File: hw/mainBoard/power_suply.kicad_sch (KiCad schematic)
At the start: 16 parts, among them Q1 NMOS, Q2 NMOS, U2 LM5148RGYR

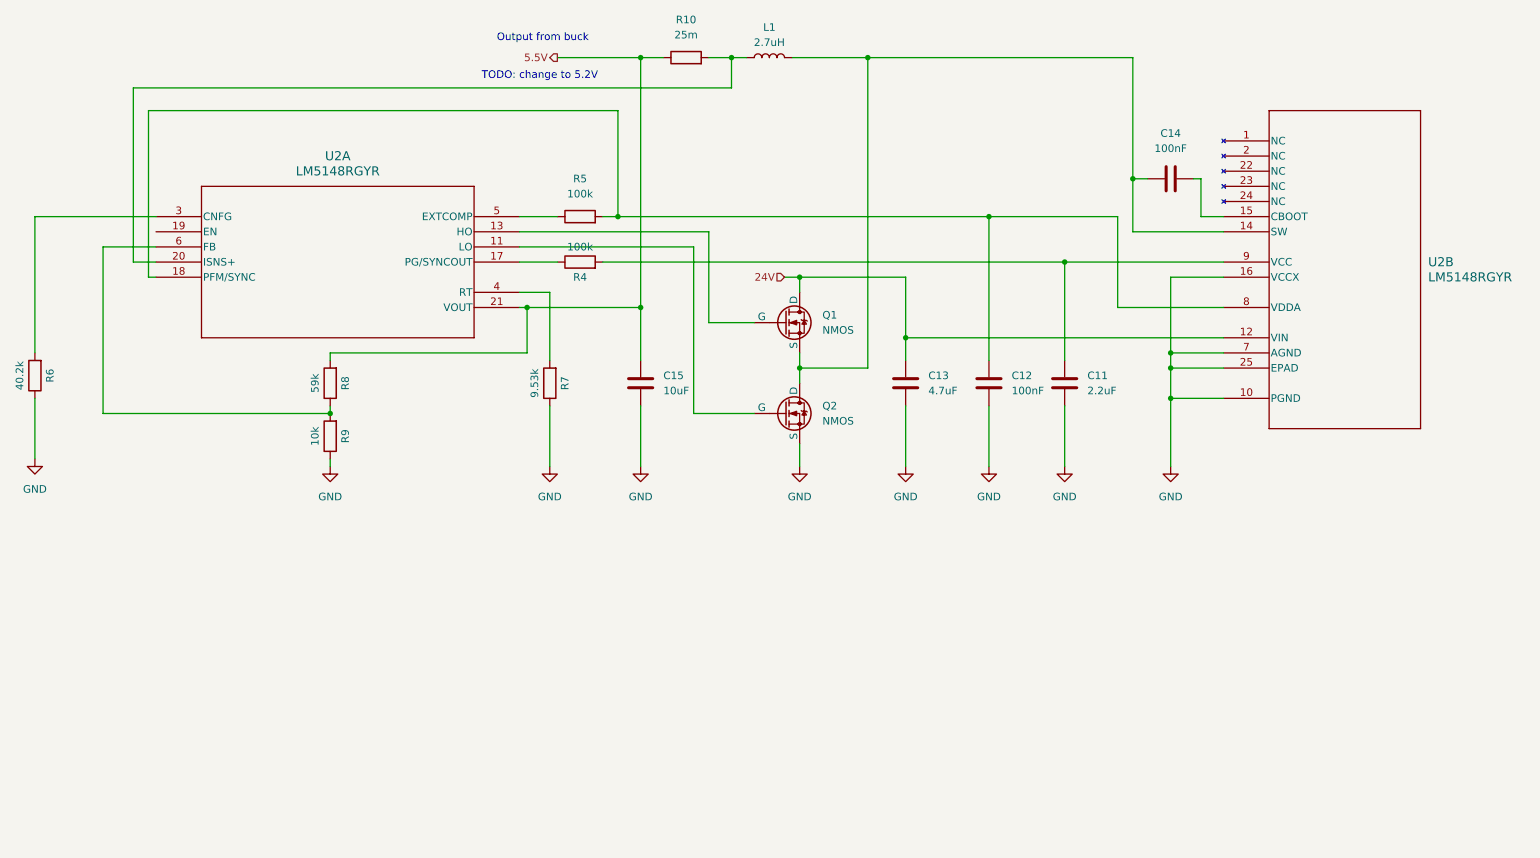
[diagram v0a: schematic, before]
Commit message: schematka
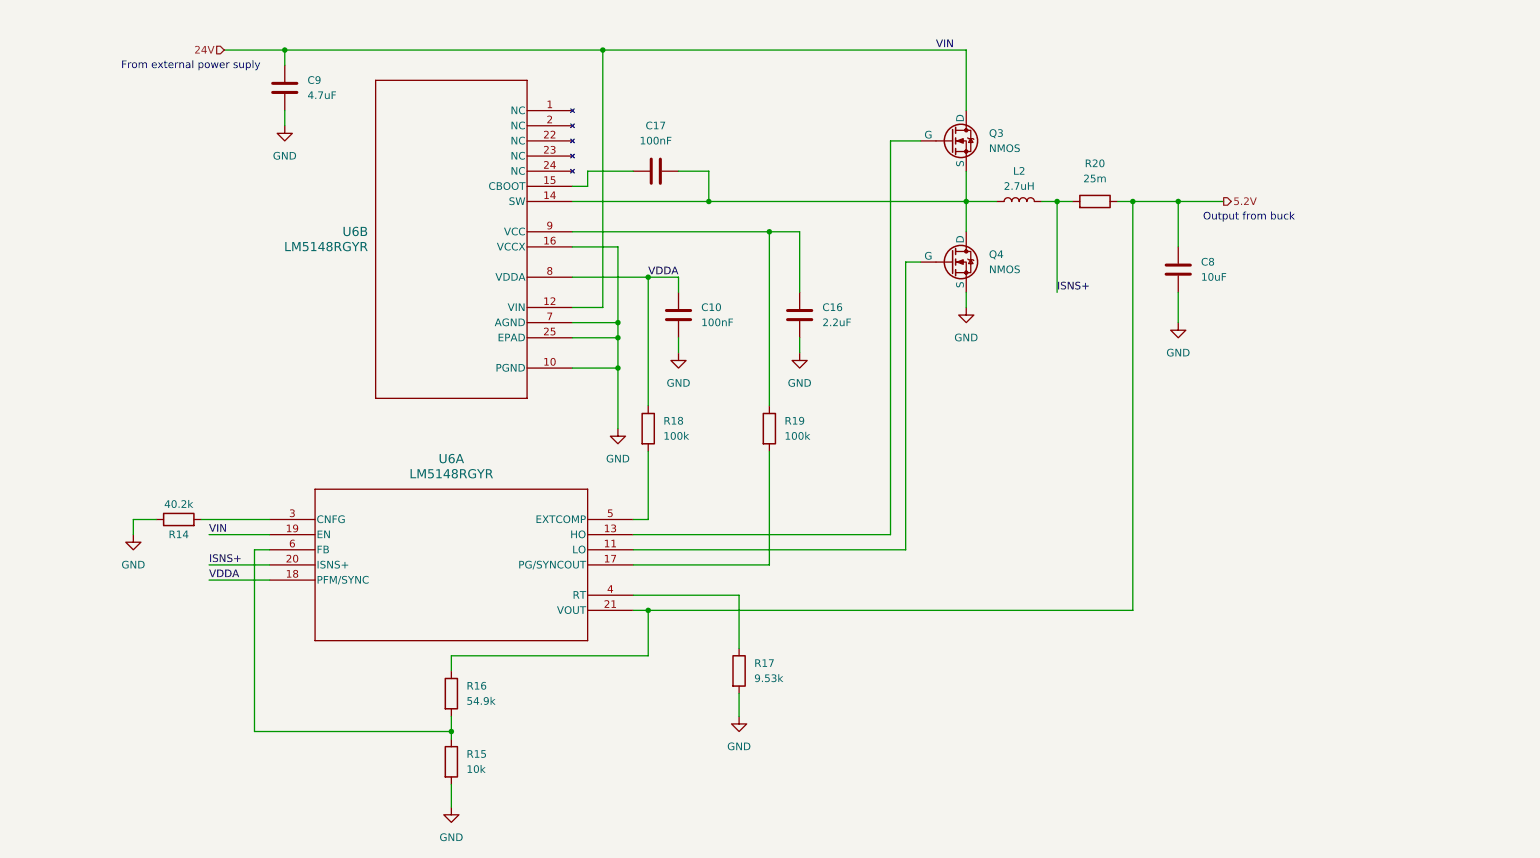
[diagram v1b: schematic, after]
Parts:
- removed C11: 2.2uF, symbol Device:C
- removed C12, C14: 100nF, symbol Device:C
- removed C13: 4.7uF, symbol Device:C
- removed C15: 10uF, symbol Device:C
- removed L1: 2.7uH, symbol Device:L
- removed Q1, Q2: NMOS, symbol Simulation_SPICE:NMOS
- removed R10: 25m, symbol Device:R
- removed R4, R5: 100k, symbol Device:R
- removed R6: 40.2k, symbol Device:R
- removed R7: 9.53k, symbol Device:R
- removed R8: 59k, symbol Device:R
- removed R9: 10k, symbol Device:R
- removed U2: LM5148RGYR, VQFN24_RGY_TEX, symbol LM5148:LM5148RGYR
- added C10, C17: 100nF, symbol Device:C
- added C16: 2.2uF, symbol Device:C
- added C8: 10uF, symbol Device:C
- added C9: 4.7uF, symbol Device:C
- added L2: 2.7uH, symbol Device:L
- added Q3, Q4: NMOS, symbol Simulation_SPICE:NMOS
- added R14: 40.2k, symbol Device:R
- added R15: 10k, symbol Device:R
- added R16: 54.9k, symbol Device:R
- added R17: 9.53k, symbol Device:R
- added R18, R19: 100k, symbol Device:R
- added R20: 25m, symbol Device:R
- added U6: LM5148RGYR, VQFN24_RGY_TEX, symbol LM5148:LM5148RGYR
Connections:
- net 24V: now also C9.1, Q3.1 (D), U6.12 (VIN), U6.19 (EN)
- net GND: now also C10.2, C16.2, C8.2, C9.2, Q4.3 (S), R14.1, R15.2, R17.2, U6.10 (PGND), U6.16 (VCCX), U6.25 (EPAD), U6.7 (AGND)
- new net: C16.1, R19.1, U6.9 (VCC)
- new net: R17.1, U6.4 (RT)
- new net: C17.2, L2.2, Q3.3 (S), Q4.1 (D), U6.14 (SW)
- new net: C17.1, U6.15 (CBOOT)
- new net: R18.2, U6.5 (EXTCOMP)
- new net: Q4.2 (G), U6.11 (LO)
- new net: Q3.2 (G), U6.13 (HO)
- new net: R19.2, U6.17 (PG/SYNCOUT)
- new net: R14.2, U6.3 (CNFG)
- new net: R15.1, R16.2, U6.6 (FB)
- new net 5.2V: C8.1, R16.1, R20.1, U6.21 (VOUT)
- new net ISNS+: L2.1, R20.2, U6.20 (ISNS+)
- new net VDDA: C10.1, R18.1, U6.18 (PFM/SYNC), U6.8 (VDDA)
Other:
- note added: "From external power suply"
- note removed: "TODO: change to 5.2V"
